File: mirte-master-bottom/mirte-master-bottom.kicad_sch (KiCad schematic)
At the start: 13 parts, among them J13 oled_conn, J6 ledstrip, Q1 DMG2305UX

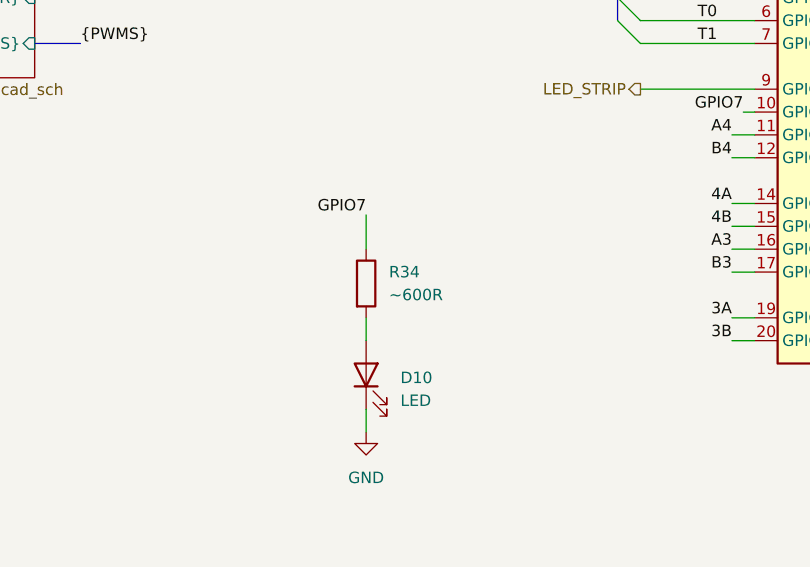
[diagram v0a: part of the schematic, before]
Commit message: mmv3 ordered pcb 2025-11-21
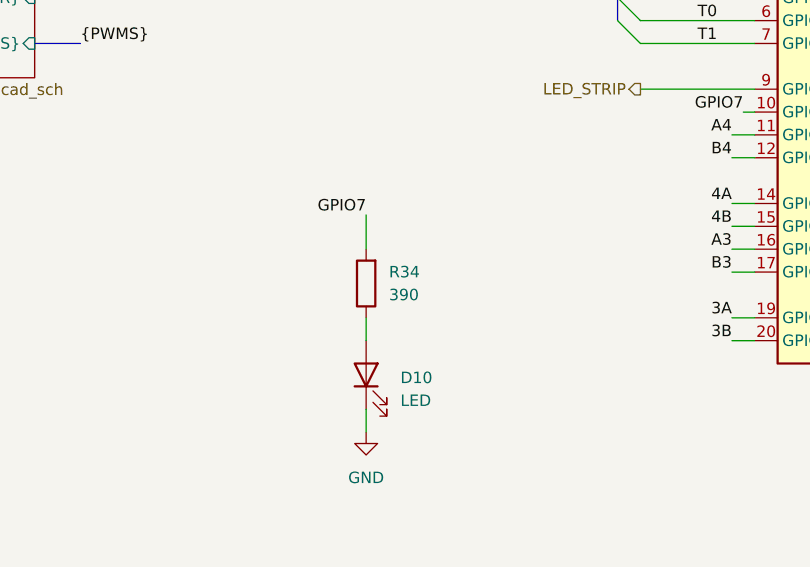
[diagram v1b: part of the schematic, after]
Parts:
- H1, H2, H3, H4: footprint MountingHole:MountingHole_3.2mm_M3_DIN965_Pad -> MountingHole:MountingHole_4.3mm_M4_DIN965_Pad
- R34: value ~600R -> 390
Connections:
- net GPIO7: now also R34.2; no longer R34.1
- net at D10.2 (A): now also R34.1; no longer R34.2
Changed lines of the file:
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@@
 			)
 		)
-		(property "Footprint" "MountingHole:MountingHole_3.2mm_M3_DIN965_Pad"
+		(property "Footprint" "MountingHole:MountingHole_4.3mm_M4_DIN965_Pad"
 			(at 71.12 134.62 0)
 			(effects
@@
 			)
 		)
-		(property "Footprint" "MountingHole:MountingHole_3.2mm_M3_DIN965_Pad"
+		(property "Footprint" "MountingHole:MountingHole_4.3mm_M4_DIN965_Pad"
 			(at 71.12 143.51 0)
 			(effects
@@
 			)
 		)
-		(property "Footprint" "MountingHole:MountingHole_3.2mm_M3_DIN965_Pad"
+		(property "Footprint" "MountingHole:MountingHole_4.3mm_M4_DIN965_Pad"
 			(at 90.17 134.62 0)
 			(effects
@@
 	(symbol
 		(lib_id "Device:R")
-		(at 162.56 130.81 0)
-		(unit 1)
-		(exclude_from_sim no)
-		(in_bom yes)
-		(on_board yes)
-		(dnp no)
-		(fields_autoplaced yes)
+		(at 162.56 130.81 180)
+		(unit 1)
+		(exclude_from_sim no)
+		(in_bom yes)
+		(on_board yes)
+		(dnp no)
 		(property "Reference" "R34"
 			(at 165.1 129.5399 0)
@@
 					(size 1.27 1.27)
 				)
-				(justify left)
-			)
-		)
-		(property "Value" "~600R"
+				(justify right)
+			)
+		)
+		(property "Value" "390"
 			(at 165.1 132.0799 0)
 			(effects
@@
 					(size 1.27 1.27)
 				)
-				(justify left)
+				(justify right)
 			)
 		)
 		(property "Footprint" "Resistor_SMD:R_0805_2012Metric"
-			(at 160.782 130.81 90)
+			(at 164.338 130.81 90)
 			(effects
 				(font
@@
 			)
 		)
-		(property "Description" ""
+		(property "Description" "Resistor"
 			(at 162.56 130.81 0)
 			(effects
@@
 			)
 		)
-		(property "Footprint" "MountingHole:MountingHole_3.2mm_M3_DIN965_Pad"
+		(property "Footprint" "MountingHole:MountingHole_4.3mm_M4_DIN965_Pad"
 			(at 90.17 143.51 0)
 			(effects
